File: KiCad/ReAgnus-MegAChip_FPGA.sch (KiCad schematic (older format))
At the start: 8 parts, among them J1 Conn_02x02_Odd_Even, J2 Conn_02x05_Odd_Even, U10 AS4C4M16SA, U11 74LVC245A, U7 GW1N-UV9LQ144, X1 SG-8002CA

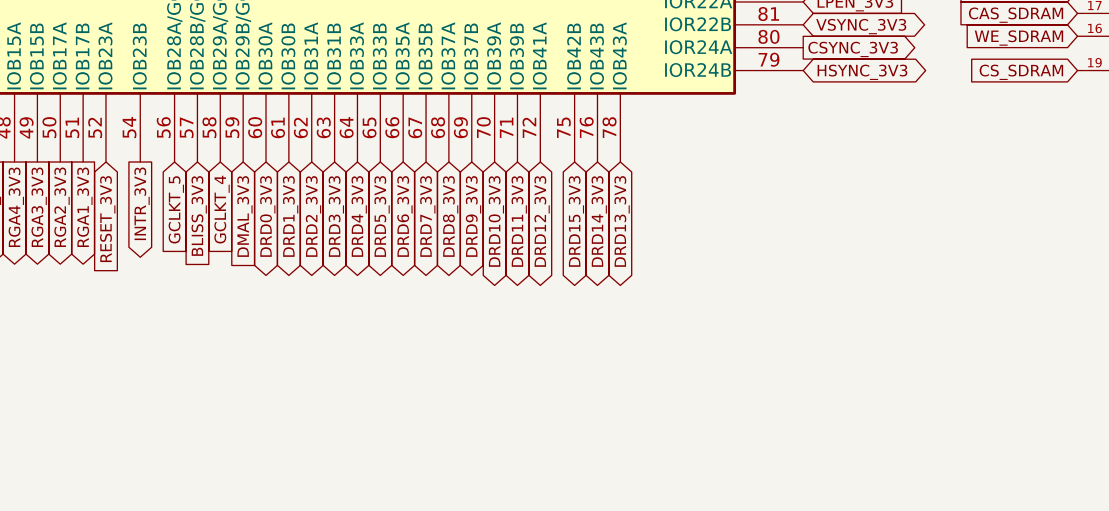
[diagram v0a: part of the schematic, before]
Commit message: more routing and placing components
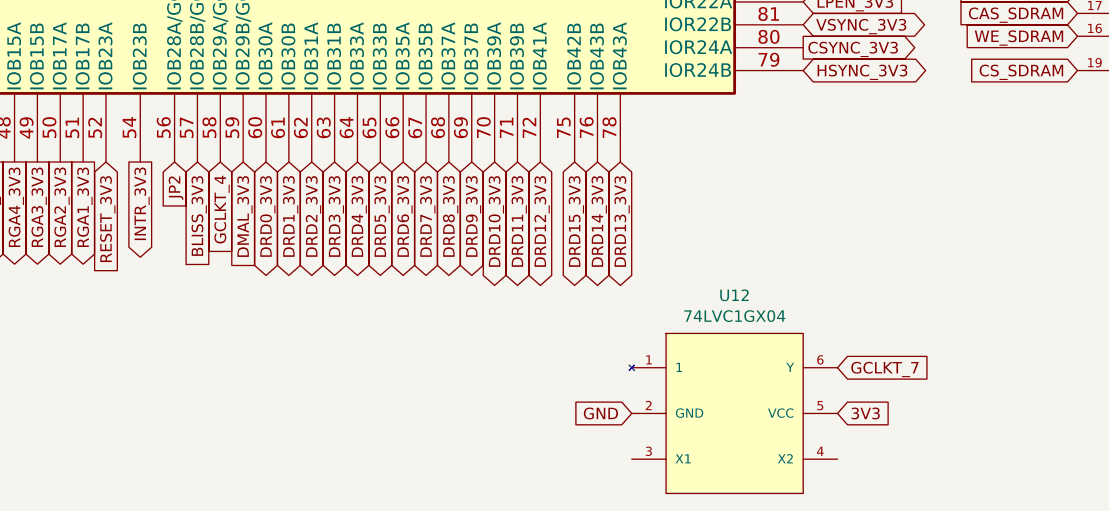
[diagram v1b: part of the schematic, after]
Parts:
- added U12: 74LVC1GX04, Package_SO:TSOP-6_1.65x3.05mm_P0.95mm, symbol ReAgnus-MegAChip:74LVC1GX04
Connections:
- net GCLKT_5 is gone; now on net JP2: U7.56 (IOB28A/GCLKT_5)
- net 3V3: now also U12.5 (VCC)
- net GCLKT_7: now also U12.6 (Y)
- net GND: now also U12.2 (GND)
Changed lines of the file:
@@
 Text GLabel 1300 3100 0    50   Input ~ 0
 GCLKT_7
-Text GLabel 3450 5950 3    50   Input ~ 0
-GCLKT_5
 Text GLabel 3650 5950 3    50   Input ~ 0
 GCLKT_4
@@
 NoConn ~ 10950 4600
 NoConn ~ 10950 4700
+$Comp
+L ReAgnus-MegAChip:74LVC1GX04 U12
+U 1 1 637F9038
+P 5900 7050
+F 0 "U12" H 5900 7565 50  0000 C CNN
+F 1 "74LVC1GX04" H 5900 7474 50  0000 C CNN
+F 2 "Package_SO:TSOP-6_1.65x3.05mm_P0.95mm" H 6400 8000 50  0001 C CNN
+F 3 "https://www.mouser.se/datasheet/2/916/74LVC1GX04-2937637.pdf" H 6400 8000 50  0001 C CNN
+	1    5900 7050
+	1    0    0    -1
+$EndComp
+Text GLabel 5450 7050 0    50   Input ~ 0
+GND
+Text GLabel 6350 7050 2    50   Input ~ 0
+3V3
+Text GLabel 6350 6850 2    50   Input ~ 0
+GCLKT_7
+Text GLabel 3450 5950 3    50   Input ~ 0
+JP2
 $EndSCHEMATC
